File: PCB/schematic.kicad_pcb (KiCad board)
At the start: 2 copper layers, 20 x 100 mm, 7 parts, among them SW1 SW_Push, SW2 SW_Push, SW3 SW_Push, SW4 SW_Push, U1 XIAO-RP2040-DIP

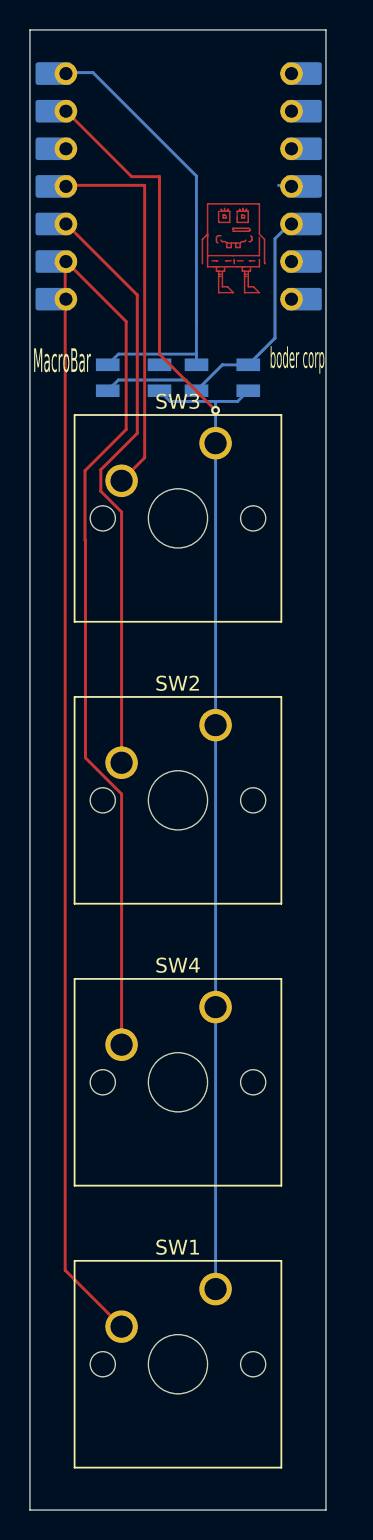
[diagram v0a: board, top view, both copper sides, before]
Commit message: s
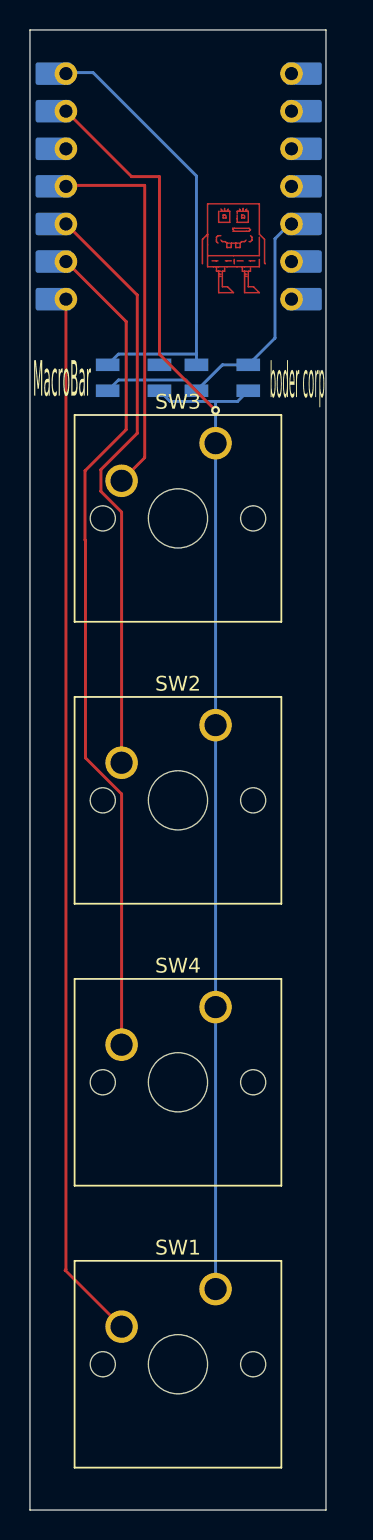
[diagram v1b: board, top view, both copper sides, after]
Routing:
- net Net-(U1-GPIO1/RX): track 72.9 -> 71.0 mm
- net unconnected-(U1-GPIO29/ADC3/A3-Pad4): track 0.82 -> 0.00 mm
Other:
- board text added: "xiao here"
